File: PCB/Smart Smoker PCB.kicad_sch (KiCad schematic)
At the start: 1 part

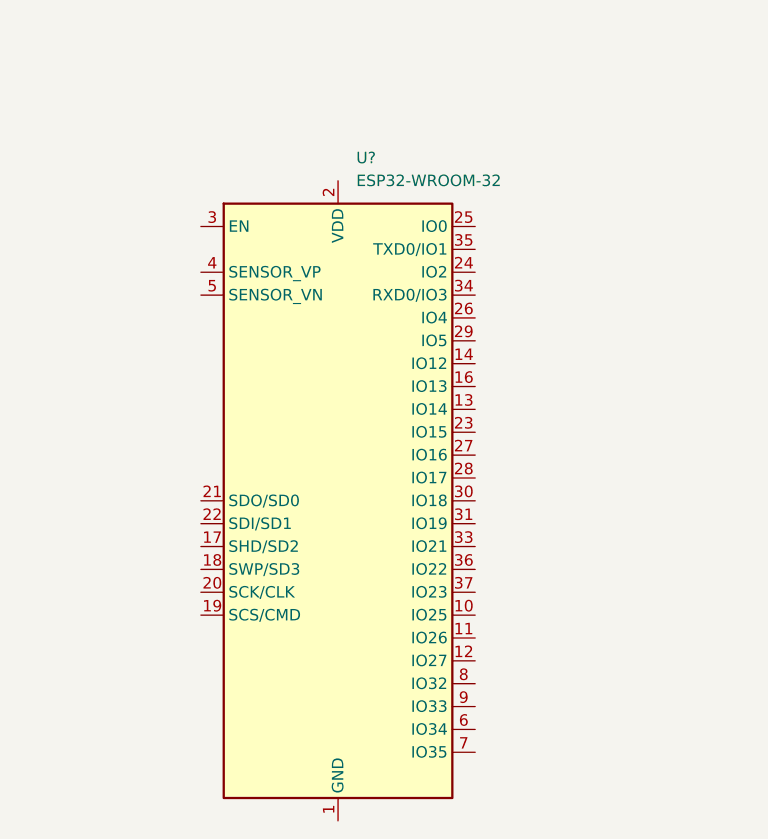
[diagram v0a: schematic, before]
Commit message: Added ESP32 board pcb files
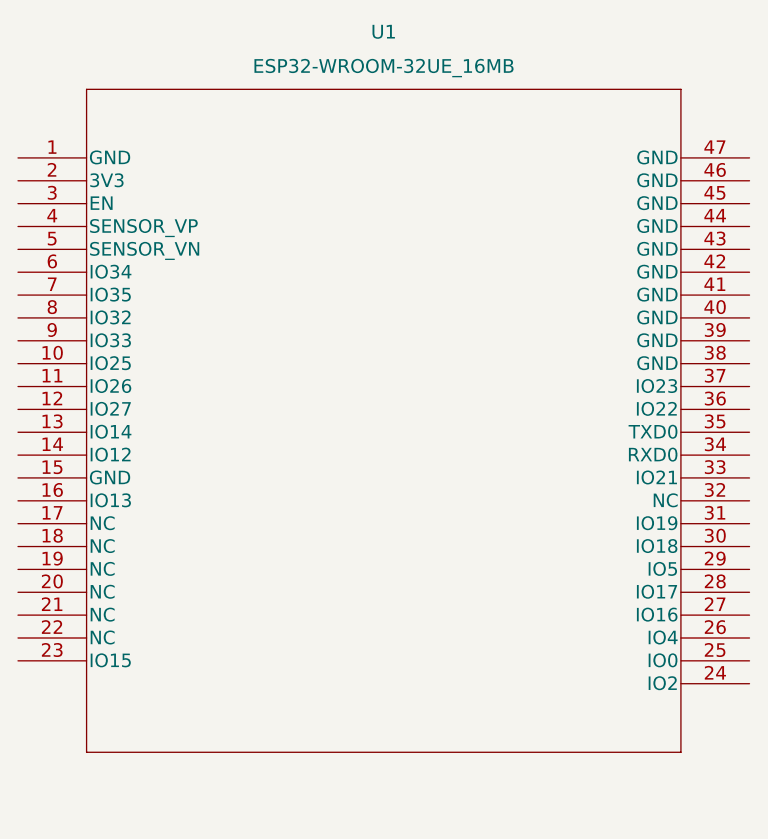
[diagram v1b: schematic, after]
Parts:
- removed U?: ESP32-WROOM-32, RF_Module:ESP32-WROOM-32, symbol RF_Module:ESP32-WROOM-32
- added U1: ESP32-WROOM-32UE_16MB, Customs Smoker:ESP32-WROOM-32UE 16MB, symbol ESP32-WROOM-32UE:ESP32-WROOM-32UE_16MB
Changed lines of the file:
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@@
 (kicad_sch (version 20211123) (generator eeschema)
   (paper "A4")
-  (symbol (lib_id "RF_Module:ESP32-WROOM-32") (at 135.89 101.6 0) (unit 1)
+  (symbol (lib_id "ESP32-WROOM-32UE:ESP32-WROOM-32UE_16MB") (at 100.33 63.5 0) (unit 1)
     (in_bom yes) (on_board yes) (fields_autoplaced)
-    (property "Reference" "U?" (id 0) (at 137.9094 63.5 0)
-      (effects (font (size 1.27 1.27)) (justify left))
+    (property "Reference" "U1" (id 0) (at 140.97 49.53 0)
+      (effects (font (size 1.524 1.524)))
     )
-    (property "Value" "ESP32-WROOM-32" (id 1) (at 137.9094 66.04 0)
-      (effects (font (size 1.27 1.27)) (justify left))
+    (property "Value" "ESP32-WROOM-32UE_16MB" (id 1) (at 140.97 53.34 0)
+      (effects (font (size 1.524 1.524)))
     )
-    (property "Footprint" "RF_Module:ESP32-WROOM-32" (id 2) (at 135.89 139.7 0)
+    (property "Footprint" "Customs Smoker:ESP32-WROOM-32UE 16MB" (id 2) (at 140.97 54.864 0)
+      (effects (font (size 1.524 1.524)) hide)
+    )
+    (property "Datasheet" "" (id 3) (at 100.33 63.5 0)
+      (effects (font (size 1.524 1.524)) hide)
+    )
+    (property "Manufacturer" "Espressif Systems" (id 4) (at 100.33 63.5 0)
       (effects (font (size 1.27 1.27)) hide)
     )
-    (property "Datasheet" "https://www.espressif.com/sites/default/files/documentation/esp32-wroom-32_datasheet_en.pdf" (id 3) (at 128.27 100.33 0)
+    (property "Manufacturer Part Number" "ESP32-WROOM-32UE-N8" (id 5) (at 100.33 63.5 0)
+      (effects (font (size 1.27 1.27)) hide)
+    )
+    (property "Vendor" "Digikey" (id 6) (at 100.33 63.5 0)
+      (effects (font (size 1.27 1.27)) hide)
+    )
+    (property "Vendor Part Number" "1965-ESP32-WROOM-32UE-N8CT-ND" (id 7) (at 100.33 63.5 0)
       (effects (font (size 1.27 1.27)) hide)
     )
@@
     (pin "39")
     (pin "4")
+    (pin "40")
+    (pin "41")
+    (pin "42")
+    (pin "43")
+    (pin "44")
+    (pin "45")
+    (pin "46")
+    (pin "47")
     (pin "5")
     (pin "6")
@@
   )
   (symbol_instances
-    (path "/4a6f9f76-50d6-4ae4-86e0-fc7dc15a31cd"
-      (reference "U?") (unit 1) (value "ESP32-WROOM-32") (footprint "RF_Module:ESP32-WROOM-32")
+    (path "/80a7e135-8f94-43f8-93fb-5e5903019107"
+      (reference "U1") (unit 1) (value "ESP32-WROOM-32UE_16MB") (footprint "Customs Smoker:ESP32-WROOM-32UE 16MB")
     )
   )
